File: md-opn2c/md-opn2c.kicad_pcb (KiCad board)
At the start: 2 copper layers, 53.1 x 29.4 mm, 41 parts, among them U1 TL072, U2 74HCT08, U3 YM3438

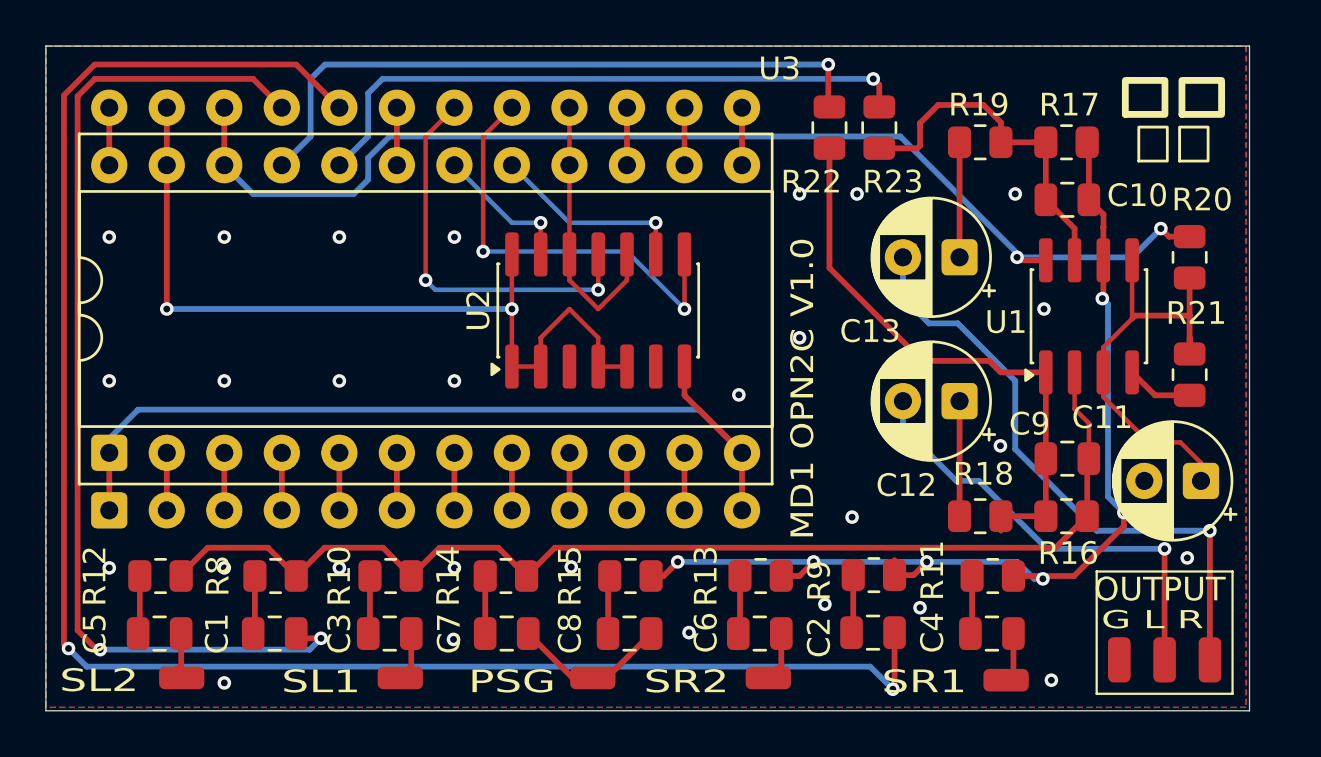
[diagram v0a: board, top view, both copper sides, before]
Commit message: little tweaks
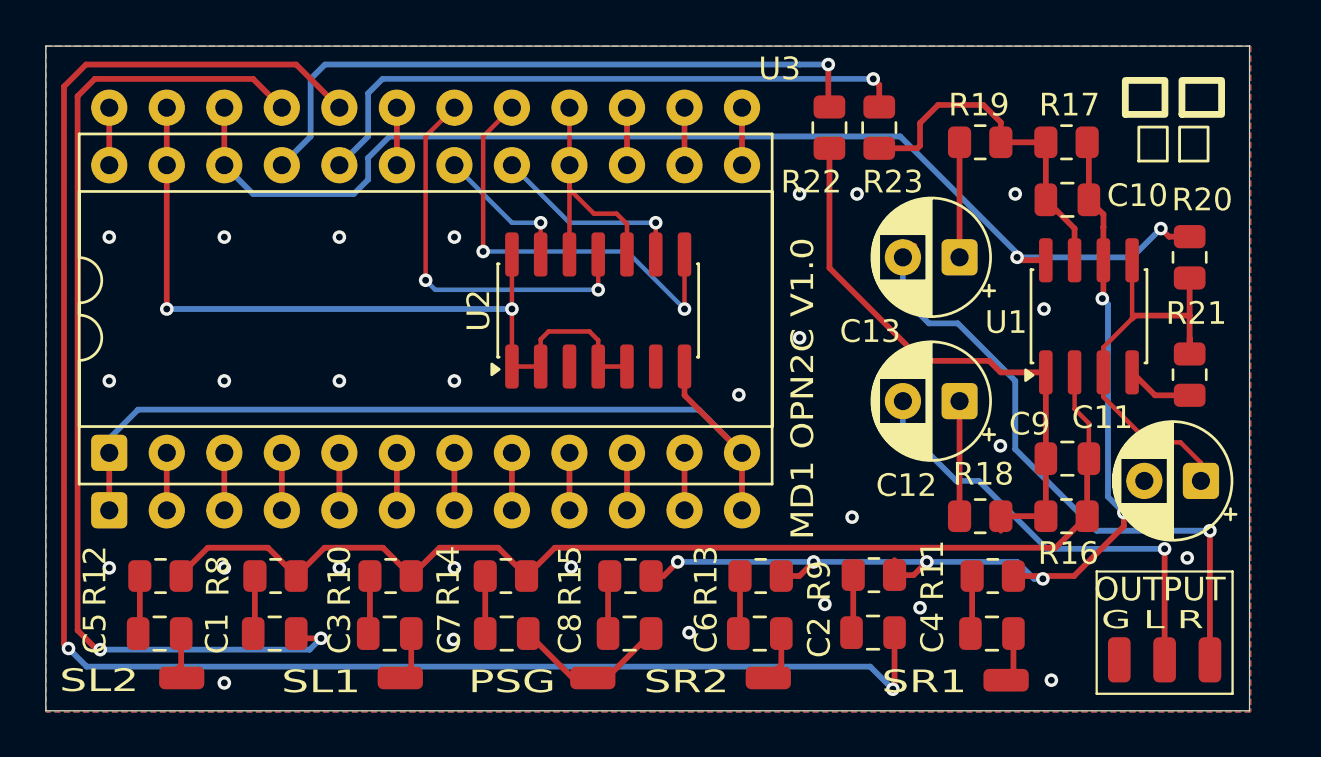
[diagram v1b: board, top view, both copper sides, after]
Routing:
- net VCC: track 37.8 -> 36.8 mm
